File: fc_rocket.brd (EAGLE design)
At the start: 88.6 x 63.5 mm, 31 parts, among them IC1 7805TV, J1 1X2-3.5MM, J2 1X2-3.5MM, J3 1X2-3.5MM, J4 1X2-3.5MM, J5 1X2-3.5MM, J6 1X2-3.5MM, U2 GY-521MPU6050

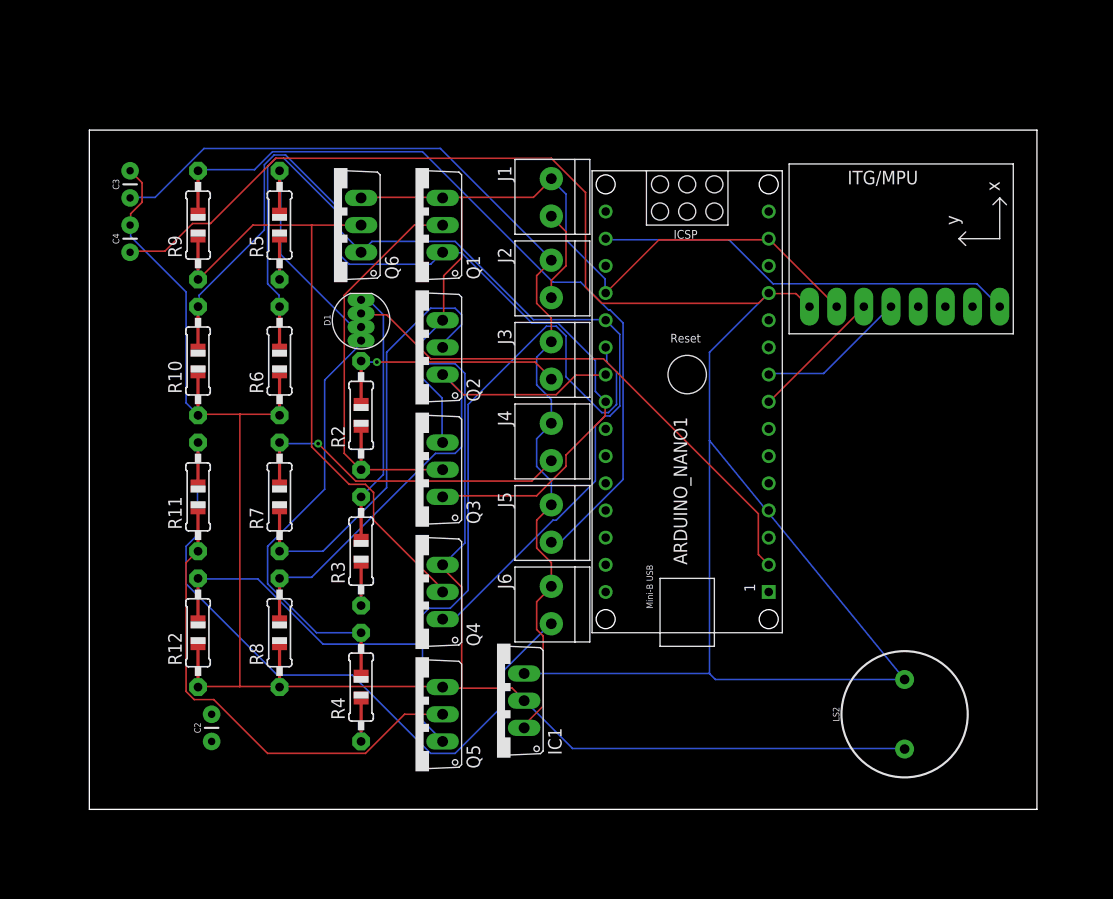
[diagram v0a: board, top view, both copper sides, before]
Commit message: finised auto router
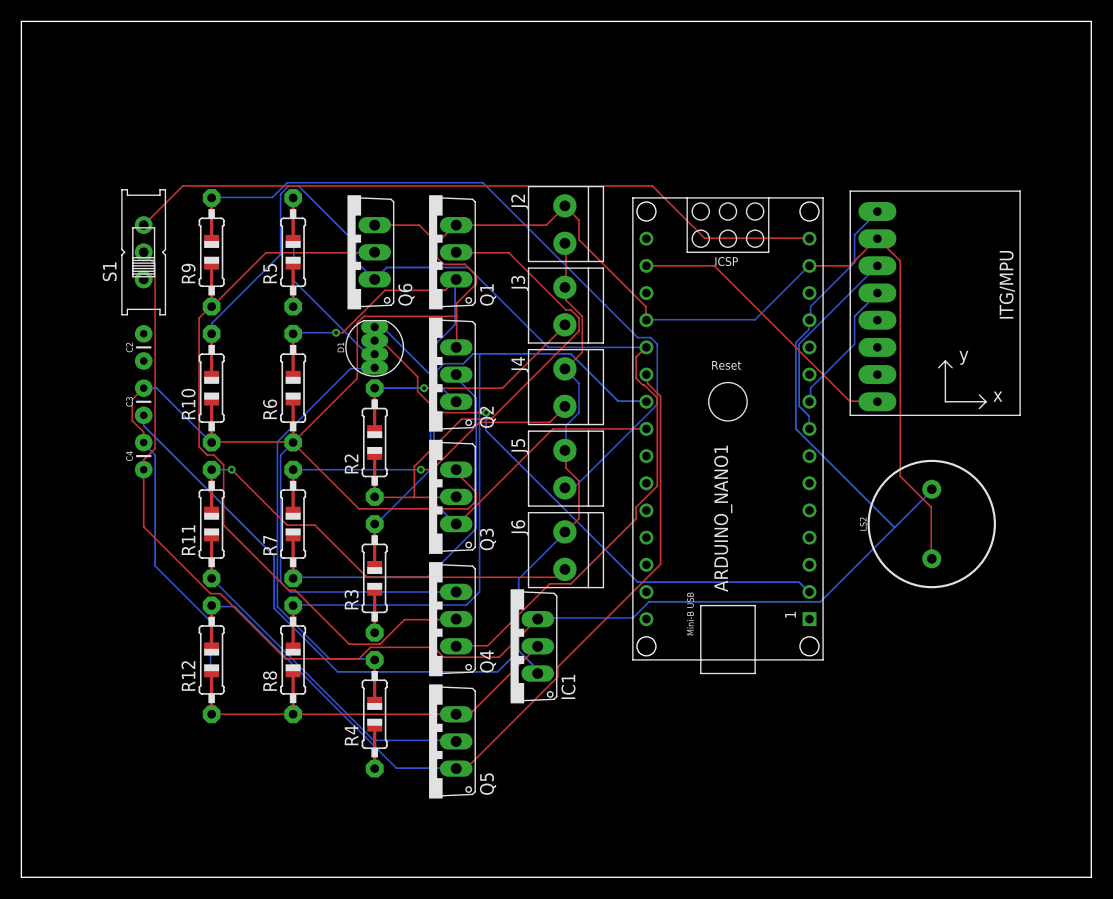
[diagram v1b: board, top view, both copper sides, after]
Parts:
- removed J1: 1X2-3.5MM, adafruit:1X2-3.5MM
- added S1: (no value), adafruit:EG1218
- moved C2 36.1 mm to (11.4, 49.5)
- moved C4 20.4 mm to (11.4, 39.4)
- moved C3 20.4 mm to (11.4, 44.5)
- moved LS2 18.0 mm to (85.1, 33.0)
- moved U2 10.9 mm to (88.9, 53.3), turned to 0 degrees
- moved J3 5.24 mm to (50.8, 53.3)
- moved J6 5.24 mm to (50.8, 30.5)
- moved IC1 5.24 mm to (45.7, 21.6)
- moved J2 5.24 mm to (50.8, 61.0)
- moved J4 5.24 mm to (50.8, 45.7)
- moved J5 5.24 mm to (50.8, 38.1)
- moved ARDUINO_NANO1 4.58 mm to (66.0, 44.5)
- moved Q4 2.84 mm to (38.1, 24.1)
- moved Q5 2.84 mm to (38.1, 12.7)
- moved R4 2.84 mm to (33.0, 15.2)
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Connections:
- removed net BATT+: J1.2, J2.2
- net 12V: now also J2.2; no longer J2.1
- net 5V: now also S1.P
- net GND: now also J2.1; no longer J1.1
- net VIN: now also S1.S
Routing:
- net VIN: track 0.00 -> 65.8 mm
- net 5V: track 181.4 -> 149.3 mm
- net N$12: track 61.4 -> 37.5 mm, vias 0 -> 1
- net PY2: track 46.4 -> 65.9 mm
- net GND: track 246.5 -> 264.4 mm
- net PY1: track 80.1 -> 63.5 mm, vias 0 -> 1
- net INT: track 39.5 -> 26.9 mm
- net N$13: track 41.5 -> 29.2 mm
- net PY3: track 87.3 -> 75.0 mm
- net N$7: track 36.5 -> 46.4 mm
- net N$11: track 57.6 -> 66.9 mm
- net BATT+: track 8.76 -> 0.00 mm
- net SCL: track 12.7 -> 18.7 mm
- net PY4: track 93.0 -> 98.3 mm
- net N$10: track 70.9 -> 66.0 mm
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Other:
- board size 88.6 x 63.5 mm -> 100 x 80 mm
